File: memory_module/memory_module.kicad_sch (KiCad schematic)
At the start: 82 parts, among them SW1 SW_DIP_x08, SW2 SW_DIP_x08, SW3 SW_DIP_x08, SW4 SW_DIP_x08, SW5 SW_DIP_x08, SW6 SW_DIP_x08, SW7 SW_DIP_x08, SW8 SW_DIP_x08, U1 74HC138, U2 74LS540

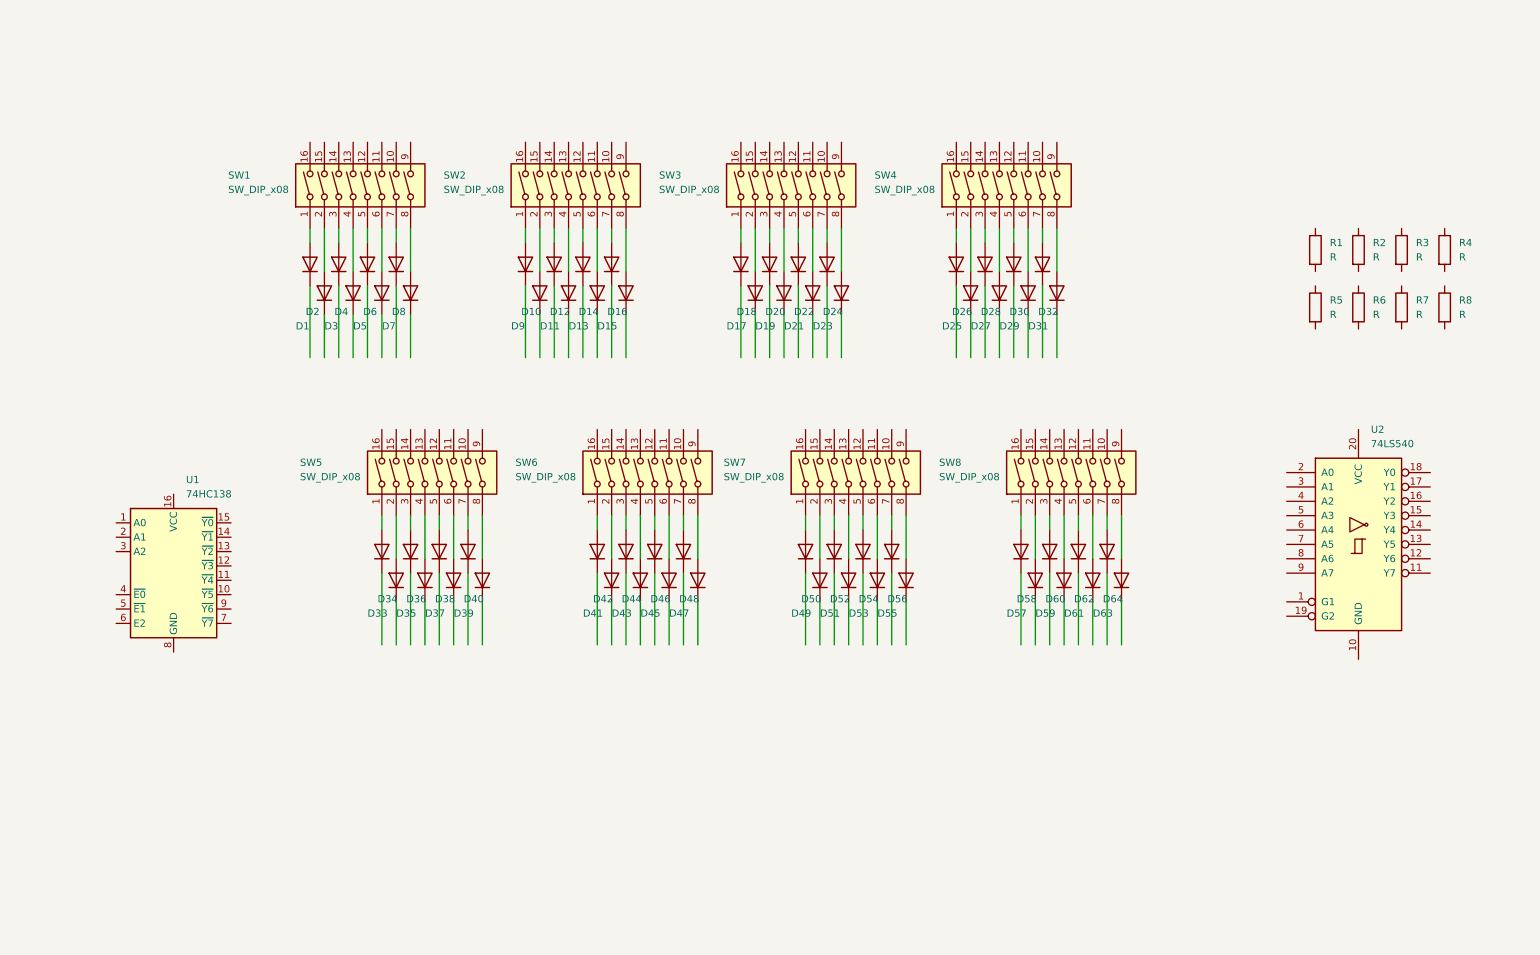
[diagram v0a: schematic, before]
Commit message: 回路図進めた
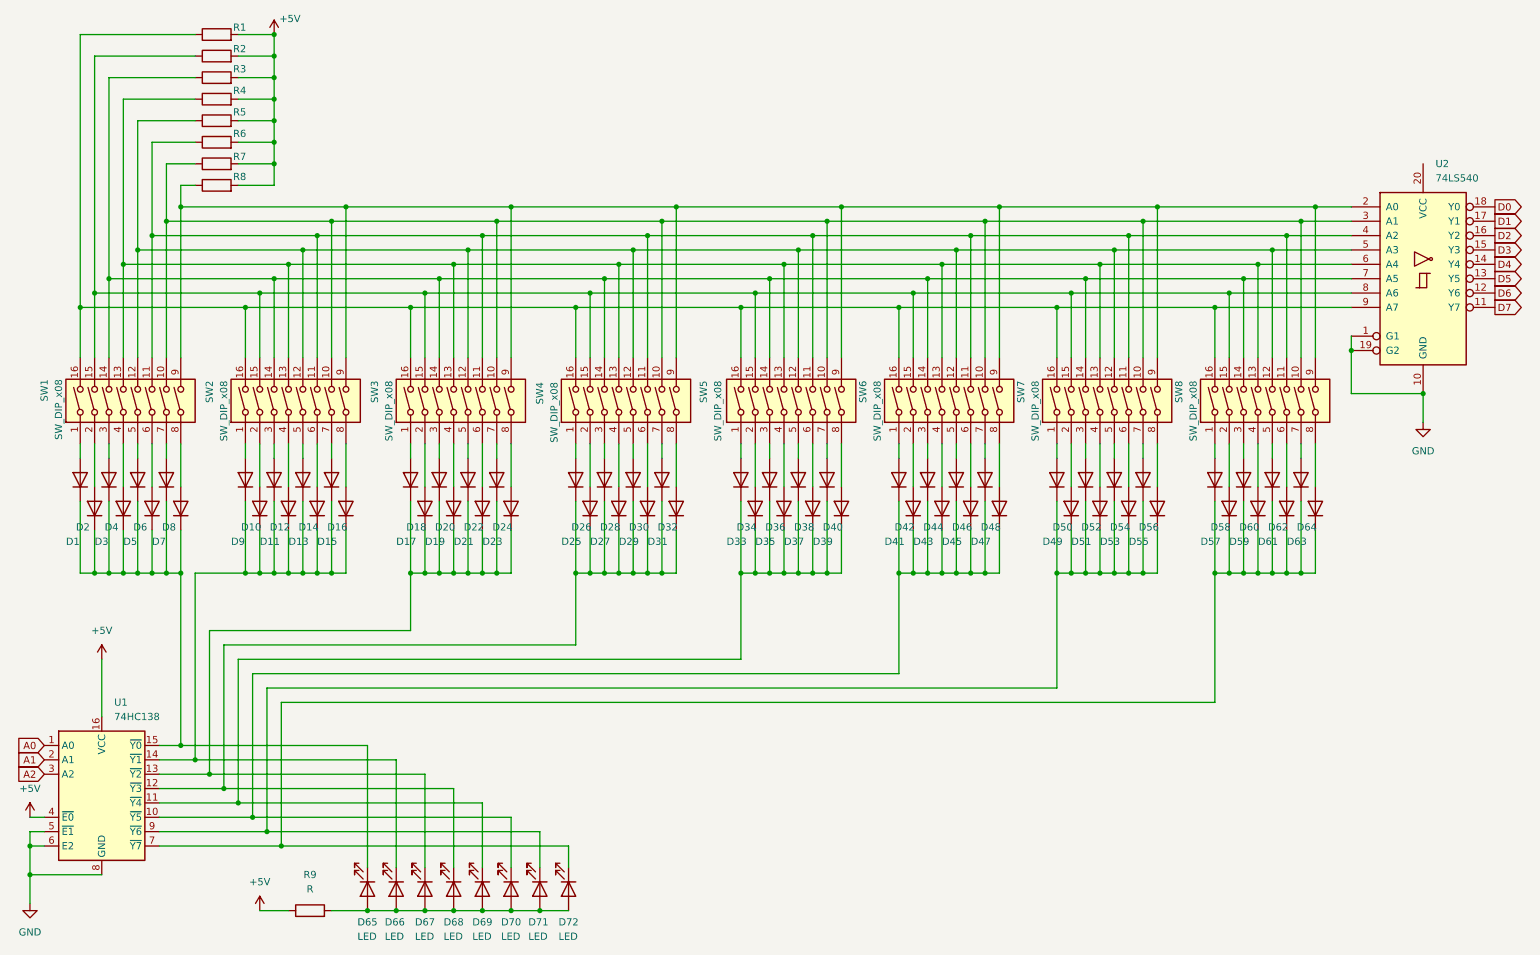
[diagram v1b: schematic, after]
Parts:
- added D65, D66, D67, D68, D69, D70, D71, D72: LED, LED_THT:LED_D3.0mm, symbol Device:LED
- added R9: R, Resistor_THT:R_Axial_DIN0207_L6.3mm_D2.5mm_P10.16mm_Horizontal, symbol Device:R
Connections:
- net at R1.1: now also SW1.16, SW2.16, SW3.16, SW4.16, SW5.16, SW6.16, SW7.16, SW8.16, U2.9 (A7)
- net +5V: now reaches R1.2
- net +5V: now also R2.2, R3.2, R4.2, R5.2, R6.2, R7.2, R8.2, U1.16 (VCC), U1.4 (~{E0}), R9.1
- net at D13.1 (K): now also D10.1 (K), D11.1 (K), D12.1 (K), D14.1 (K), D15.1 (K), D16.1 (K), D9.1 (K), U1.14 (~{Y1}), D66.1 (K)
- net at D56.1 (K): now also D49.1 (K), D50.1 (K), D51.1 (K), D52.1 (K), D53.1 (K), D54.1 (K), D55.1 (K), U1.9 (~{Y6}), D71.1 (K)
- net at D27.1 (K): now also D25.1 (K), D26.1 (K), D28.1 (K), D29.1 (K), D30.1 (K), D31.1 (K), D32.1 (K), U1.12 (~{Y3}), D68.1 (K)
- net at R4.1: now also SW1.13, SW2.13, SW3.13, SW4.13, SW5.13, SW6.13, SW7.13, SW8.13, U2.6 (A4)
- net at D17.1 (K): now also D18.1 (K), D19.1 (K), D20.1 (K), D21.1 (K), D22.1 (K), D23.1 (K), D24.1 (K), U1.13 (~{Y2}), D67.1 (K)
- net at D7.1 (K): now also D1.1 (K), D2.1 (K), D3.1 (K), D4.1 (K), D5.1 (K), D6.1 (K), D8.1 (K), U1.15 (~{Y0}), D65.1 (K)
- net at D62.1 (K): now also D57.1 (K), D58.1 (K), D59.1 (K), D60.1 (K), D61.1 (K), D63.1 (K), D64.1 (K), U1.7 (~{Y7}), D72.1 (K)
- net at R3.1: now also SW1.14, SW2.14, SW3.14, SW4.14, SW5.14, SW6.14, SW7.14, SW8.14, U2.7 (A5)
- net at D40.1 (K): now also D33.1 (K), D34.1 (K), D35.1 (K), D36.1 (K), D37.1 (K), D38.1 (K), D39.1 (K), U1.11 (~{Y4}), D69.1 (K)
- net at R5.1: now also SW1.12, SW2.12, SW3.12, SW4.12, SW5.12, SW6.12, SW7.12, SW8.12, U2.5 (A3)
- net at D41.1 (K): now also D42.1 (K), D43.1 (K), D44.1 (K), D45.1 (K), D46.1 (K), D47.1 (K), D48.1 (K), U1.10 (~{Y5}), D70.1 (K)
- net at SW8.10: now also R7.1, SW1.10, SW2.10, SW3.10, SW4.10, SW5.10, SW6.10, SW7.10, U2.3 (A1)
- net at SW8.11: now also R6.1, SW1.11, SW2.11, SW3.11, SW4.11, SW5.11, SW6.11, SW7.11, U2.4 (A2)
- net at SW8.15: now also R2.1, SW1.15, SW2.15, SW3.15, SW4.15, SW5.15, SW6.15, SW7.15, U2.8 (A6)
- net at SW8.9: now also R8.1, SW1.9, SW2.9, SW3.9, SW4.9, SW5.9, SW6.9, SW7.9, U2.2 (A0)
- net GND: now reaches U2.1 (G1)
- net GND: now also U1.5 (~{E1}), U1.6 (E2), U1.8 (GND), U2.10 (GND), U2.19 (G2)
- net D7: now reaches U2.11 (Y7)
- net D6: now reaches U2.12 (Y6)
- net D5: now reaches U2.13 (Y5)
- net D4: now reaches U2.14 (Y4)
- net D3: now reaches U2.15 (Y3)
- net D2: now reaches U2.16 (Y2)
- net D1: now reaches U2.17 (Y1)
- net D0: now reaches U2.18 (Y0)
- net A0: now reaches U1.1 (A0)
- net A1: now reaches U1.2 (A1)
- net A2: now reaches U1.3 (A2)
- new net: D65.2 (A), D66.2 (A), D67.2 (A), D68.2 (A), D69.2 (A), D70.2 (A), D71.2 (A), D72.2 (A), R9.2
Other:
- moved on the sheet: D1, D10, D11, D12, D13, D14, D15, D16, D17, D18, D19, D2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
